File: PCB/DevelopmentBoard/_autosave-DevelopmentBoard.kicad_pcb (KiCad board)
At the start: 2 copper layers, 152.4 x 76.2 mm, 45 parts, among them J2 Conn_01x04_MountingPin-Payloa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, J5 Conn_01x04_MountingPin, U1 D24V22F5_VoltageRegulator, U3 RASPBERRY_PI_3_MODEL_B+, U4 Conn_01x08_DevBoardSymbols, U6 MCP3008_ADC, U7 Conn_01x06_DevBoard_Symbols, X1 XT30, X2 XT30, X3 2mmGrove_Connector

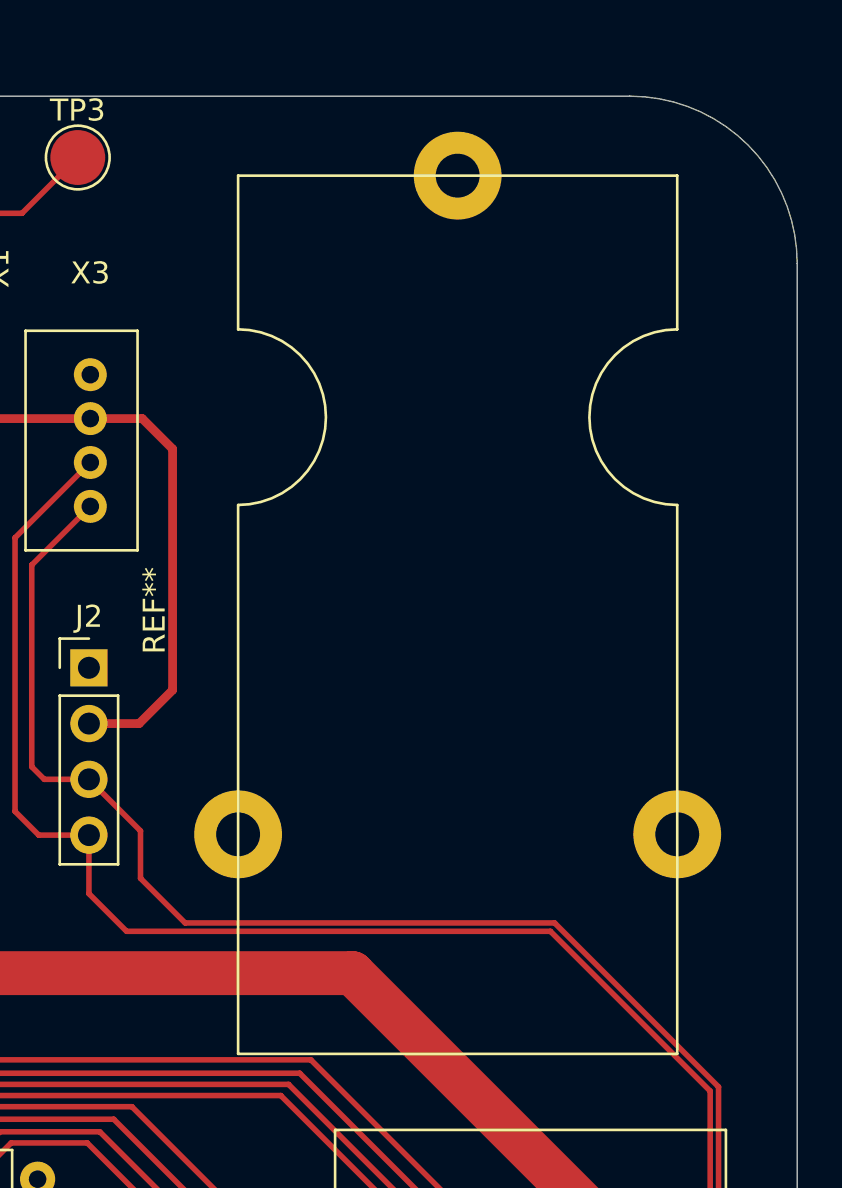
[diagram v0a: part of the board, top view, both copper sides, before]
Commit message: Overwrite files.
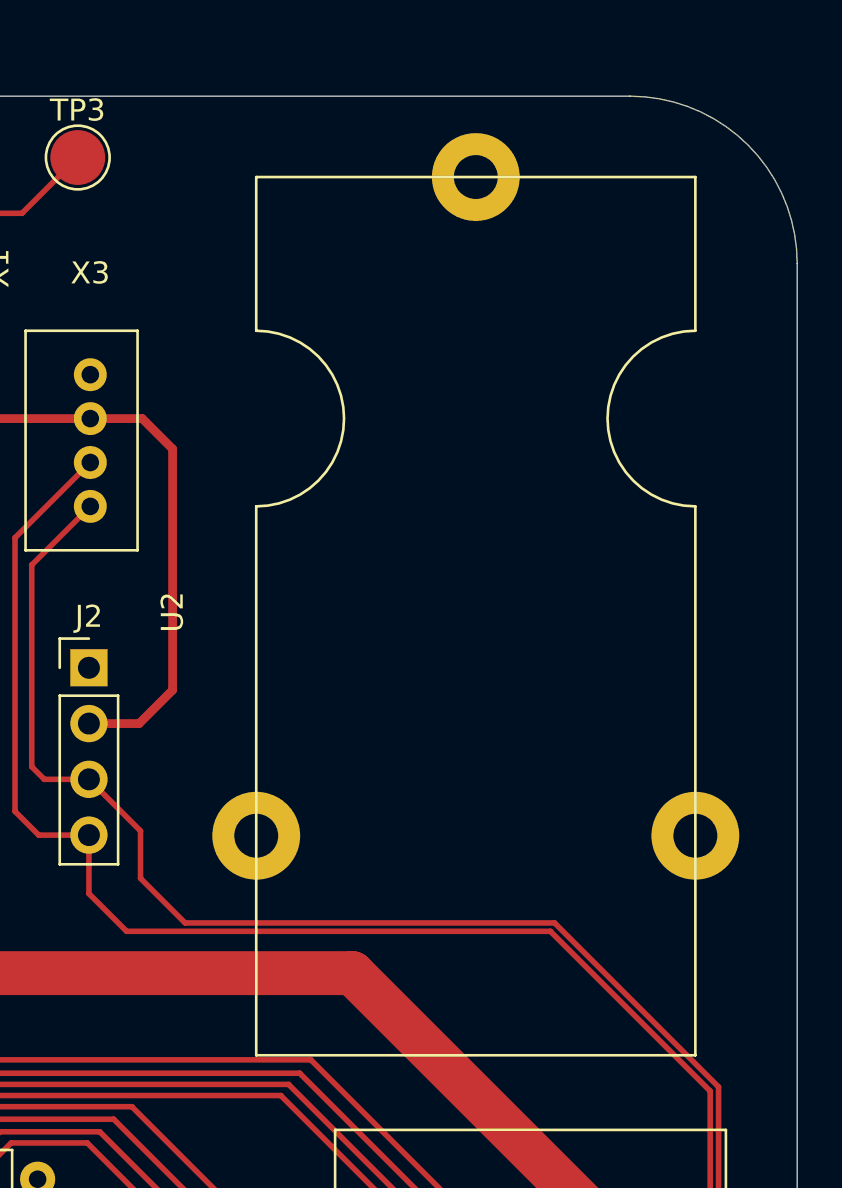
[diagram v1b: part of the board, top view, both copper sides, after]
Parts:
- removed the REF** at (199.6, 66.1)
- added U2: Barometer_Grove, DevelopmentBoard:Barometer_Grove, F.Cu at (200.5, 66.1)
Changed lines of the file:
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@@
-    )
-  )
-  (module DevelopmentBoard:Barometer_Grove (layer Front)
-    (at 199.6425 66.0655 90)
-    (fp_text reference REF** (at -19.812 -3.81 90) (layer F.SilkS)
-      (effects (font (size 1 1) (thickness 0.15)))
-    )
-    (fp_text value Barometer_Grove (at -19.05 24.384 90) (layer F.Fab)
-      (effects (font (size 1 1) (thickness 0.15)))
-    )
-    (fp_line (start -15 0) (end -40 0) (layer F.SilkS) (width 0.12))
-    (fp_line (start -15 20) (end -40 20) (layer F.SilkS) (width 0.12))
-    (fp_line (start 0 20) (end -7 20) (layer F.SilkS) (width 0.12))
-    (fp_line (start 0 0) (end 0 20) (layer F.SilkS) (width 0.12))
-    (fp_line (start -40 0) (end -40 20) (layer F.SilkS) (width 0.12))
-    (fp_line (start -7 0) (end 0 0) (layer F.SilkS) (width 0.12))
-    (fp_line (start -14.6 0) (end -14.6 -0.4) (layer F.CrtYd) (width 0.12))
-    (fp_line (start -27.734013 -0.394085) (end -14.6 -0.4) (layer F.CrtYd) (width 0.12))
-    (fp_line (start -27.734013 20.494085) (end -14.6 20.5) (layer F.CrtYd) (width 0.12))
-    (fp_line (start -14.6 20.5) (end -14.6 20) (layer F.CrtYd) (width 0.12))
-    (fp_line (start -7.4 0) (end -7.4 -0.4) (layer F.CrtYd) (width 0.12))
-    (fp_line (start -7.4 -0.4) (end 0.4 -0.4) (layer F.CrtYd) (width 0.12))
-    (fp_line (start 0.4 -0.4) (end 0.394085 7.734013) (layer F.CrtYd) (width 0.12))
-    (fp_line (start 0.394085 12.265987) (end 0.4 20.4) (layer F.CrtYd) (width 0.12))
-    (fp_line (start 0.4 20.4) (end 0.4 20.5) (layer F.CrtYd) (width 0.12))
-    (fp_line (start 0.4 20.5) (end -7.4 20.5) (layer F.CrtYd) (width 0.12))
-    (fp_line (start -7.4 20.5) (end -7.4 20) (layer F.CrtYd) (width 0.12))
-    (fp_line (start -32.265987 -0.394085) (end -40.4 -0.4) (layer F.CrtYd) (width 0.12))
-    (fp_line (start -40.4 -0.4) (end -40.4 20.4) (layer F.CrtYd) (width 0.12))
-    (fp_line (start -32.265987 20.494085) (end -40.4 20.5) (layer F.CrtYd) (width 0.12))
-    (fp_line (start -40.4 20.5) (end -40.4 20.4) (layer F.CrtYd) (width 0.12))
-    (fp_arc (start 0 10) (end 2.3 10) (angle -80.13419306) (layer F.CrtYd) (width 0.12))
-    (fp_arc (start 0 10) (end 2.3 10) (angle 80.13419306) (layer F.CrtYd) (width 0.12))
-    (fp_arc (start -11 20) (end -7.4 20) (angle -180) (layer F.CrtYd) (width 0.12))
-    (fp_arc (start -11 0) (end -14.6 0) (angle -180) (layer F.CrtYd) (width 0.12))
-    (fp_arc (start -30 0) (end -30 -2.3) (angle 80.13419306) (layer F.CrtYd) (width 0.12))
-    (fp_arc (start -11 20) (end -7 20) (angle -180) (layer F.SilkS) (width 0.12))
-    (fp_arc (start -11 0) (end -15 0) (angle -180) (layer F.SilkS) (width 0.12))
-    (fp_arc (start -30 0) (end -30 -2.3) (angle -80.13419306) (layer F.CrtYd) (width 0.12))
-    (fp_arc (start -30 20.1) (end -30 22.4) (angle -80.13419306) (layer F.CrtYd) (width 0.12))
-    (fp_arc (start -30 20.1) (end -30 22.4) (angle 80.13419306) (layer F.CrtYd) (width 0.12))
-    (pad "" thru_hole circle (at 0 10 90) (size 4 4) (drill 2) (layers *.Cu *.Mask))
-    (pad "" thru_hole circle (at -30 0 90) (size 4 4) (drill 2) (layers *.Cu *.Mask))
-    (pad "" thru_hole circle (at -30 20 90) (size 4 4) (drill 2) (layers *.Cu *.Mask))
-    (model "${KIPRJMOD}/Models/Grove Altimeter.step"
-      (offset (xyz -18.65 31.75 1.5))
-      (scale (xyz 1 1 1))
-      (rotate (xyz -90 0 0))
     )
   )
@@
     )
   )
+  (module DevelopmentBoard:Barometer_Grove (layer Front)
+    (at 200.468 66.129 90)
+    (fp_text reference U2 (at -19.812 -3.81 90) (layer F.SilkS)
+      (effects (font (size 1 1) (thickness 0.15)))
+    )
+    (fp_text value Barometer_Grove (at -19.05 24.384 90) (layer F.Fab)
+      (effects (font (size 1 1) (thickness 0.15)))
+    )
+    (fp_line (start -15 0) (end -40 0) (layer F.SilkS) (width 0.12))
+    (fp_line (start -15 20) (end -40 20) (layer F.SilkS) (width 0.12))
+    (fp_line (start 0 20) (end -7 20) (layer F.SilkS) (width 0.12))
+    (fp_line (start 0 0) (end 0 20) (layer F.SilkS) (width 0.12))
+    (fp_line (start -40 0) (end -40 20) (layer F.SilkS) (width 0.12))
+    (fp_line (start -7 0) (end 0 0) (layer F.SilkS) (width 0.12))
+    (fp_line (start -14.6 0) (end -14.6 -0.4) (layer F.CrtYd) (width 0.12))
+    (fp_line (start -27.734013 -0.394085) (end -14.6 -0.4) (layer F.CrtYd) (width 0.12))
+    (fp_line (start -27.734013 20.494085) (end -14.6 20.5) (layer F.CrtYd) (width 0.12))
+    (fp_line (start -14.6 20.5) (end -14.6 20) (layer F.CrtYd) (width 0.12))
+    (fp_line (start -7.4 0) (end -7.4 -0.4) (layer F.CrtYd) (width 0.12))
+    (fp_line (start -7.4 -0.4) (end 0.4 -0.4) (layer F.CrtYd) (width 0.12))
+    (fp_line (start 0.4 -0.4) (end 0.394085 7.734013) (layer F.CrtYd) (width 0.12))
+    (fp_line (start 0.394085 12.265987) (end 0.4 20.4) (layer F.CrtYd) (width 0.12))
+    (fp_line (start 0.4 20.4) (end 0.4 20.5) (layer F.CrtYd) (width 0.12))
+    (fp_line (start 0.4 20.5) (end -7.4 20.5) (layer F.CrtYd) (width 0.12))
+    (fp_line (start -7.4 20.5) (end -7.4 20) (layer F.CrtYd) (width 0.12))
+    (fp_line (start -32.265987 -0.394085) (end -40.4 -0.4) (layer F.CrtYd) (width 0.12))
+    (fp_line (start -40.4 -0.4) (end -40.4 20.4) (layer F.CrtYd) (width 0.12))
+    (fp_line (start -32.265987 20.494085) (end -40.4 20.5) (layer F.CrtYd) (width 0.12))
+    (fp_line (start -40.4 20.5) (end -40.4 20.4) (layer F.CrtYd) (width 0.12))
+    (fp_arc (start -30 20.1) (end -30 22.4) (angle 80.13419306) (layer F.CrtYd) (width 0.12))
+    (fp_arc (start -30 20.1) (end -30 22.4) (angle -80.13419306) (layer F.CrtYd) (width 0.12))
+    (fp_arc (start -30 0) (end -30 -2.3) (angle -80.13419306) (layer F.CrtYd) (width 0.12))
+    (fp_arc (start -11 0) (end -15 0) (angle -180) (layer F.SilkS) (width 0.12))
+    (fp_arc (start -11 20) (end -7 20) (angle -180) (layer F.SilkS) (width 0.12))
+    (fp_arc (start -30 0) (end -30 -2.3) (angle 80.13419306) (layer F.CrtYd) (width 0.12))
+    (fp_arc (start -11 0) (end -14.6 0) (angle -180) (layer F.CrtYd) (width 0.12))
+    (fp_arc (start -11 20) (end -7.4 20) (angle -180) (layer F.CrtYd) (width 0.12))
+    (fp_arc (start 0 10) (end 2.3 10) (angle 80.13419306) (layer F.CrtYd) (width 0.12))
+    (fp_arc (start 0 10) (end 2.3 10) (angle -80.13419306) (layer F.CrtYd) (width 0.12))
+    (pad "" thru_hole circle (at -30 20 90) (size 4 4) (drill 2) (layers *.Cu *.Mask))
+    (pad "" thru_hole circle (at -30 0 90) (size 4 4) (drill 2) (layers *.Cu *.Mask))
+    (pad "" thru_hole circle (at 0 10 90) (size 4 4) (drill 2) (layers *.Cu *.Mask))
+    (model "${KIPRJMOD}/Models/Grove Altimeter.step"
+      (offset (xyz -18.65 31.75 1.5))
+      (scale (xyz 1 1 1))
+      (rotate (xyz -90 0 0))
+    )
+  )
